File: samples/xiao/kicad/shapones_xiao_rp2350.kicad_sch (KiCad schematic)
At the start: 44 parts, among them Q1 PMOS, Q4 NMOS, SW1 POWER, SW10 MENU, SW2 A, SW3 B, SW4 SELECT, SW5 START, SW6 UP, SW7 DOWN, SW8 LEFT, SW9 RIGHT, U1 XIAO RP2350, U2 PCA9555D, U4 1.54''IPS-240x240, U5 TFCard, U6 74AHC1G04W5, U7 HT82V73A

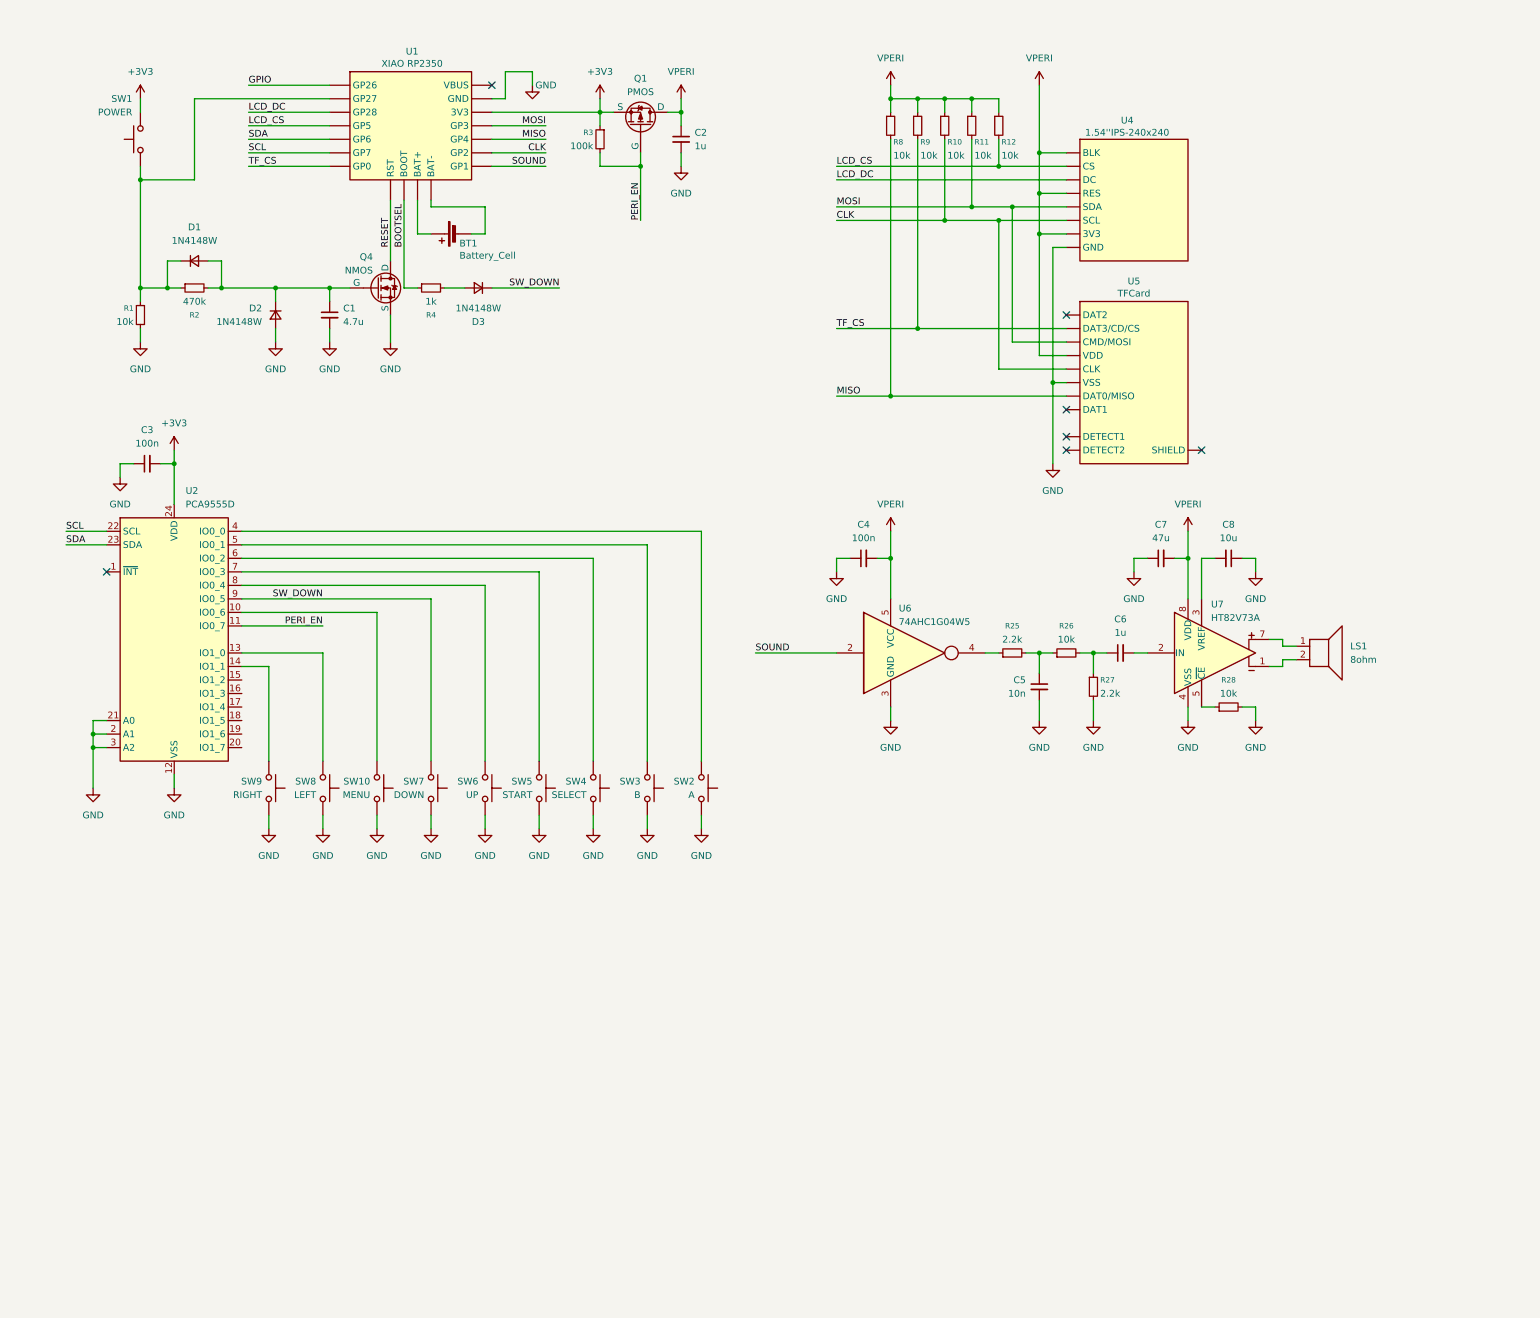
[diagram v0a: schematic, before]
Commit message: wip: PCB layout
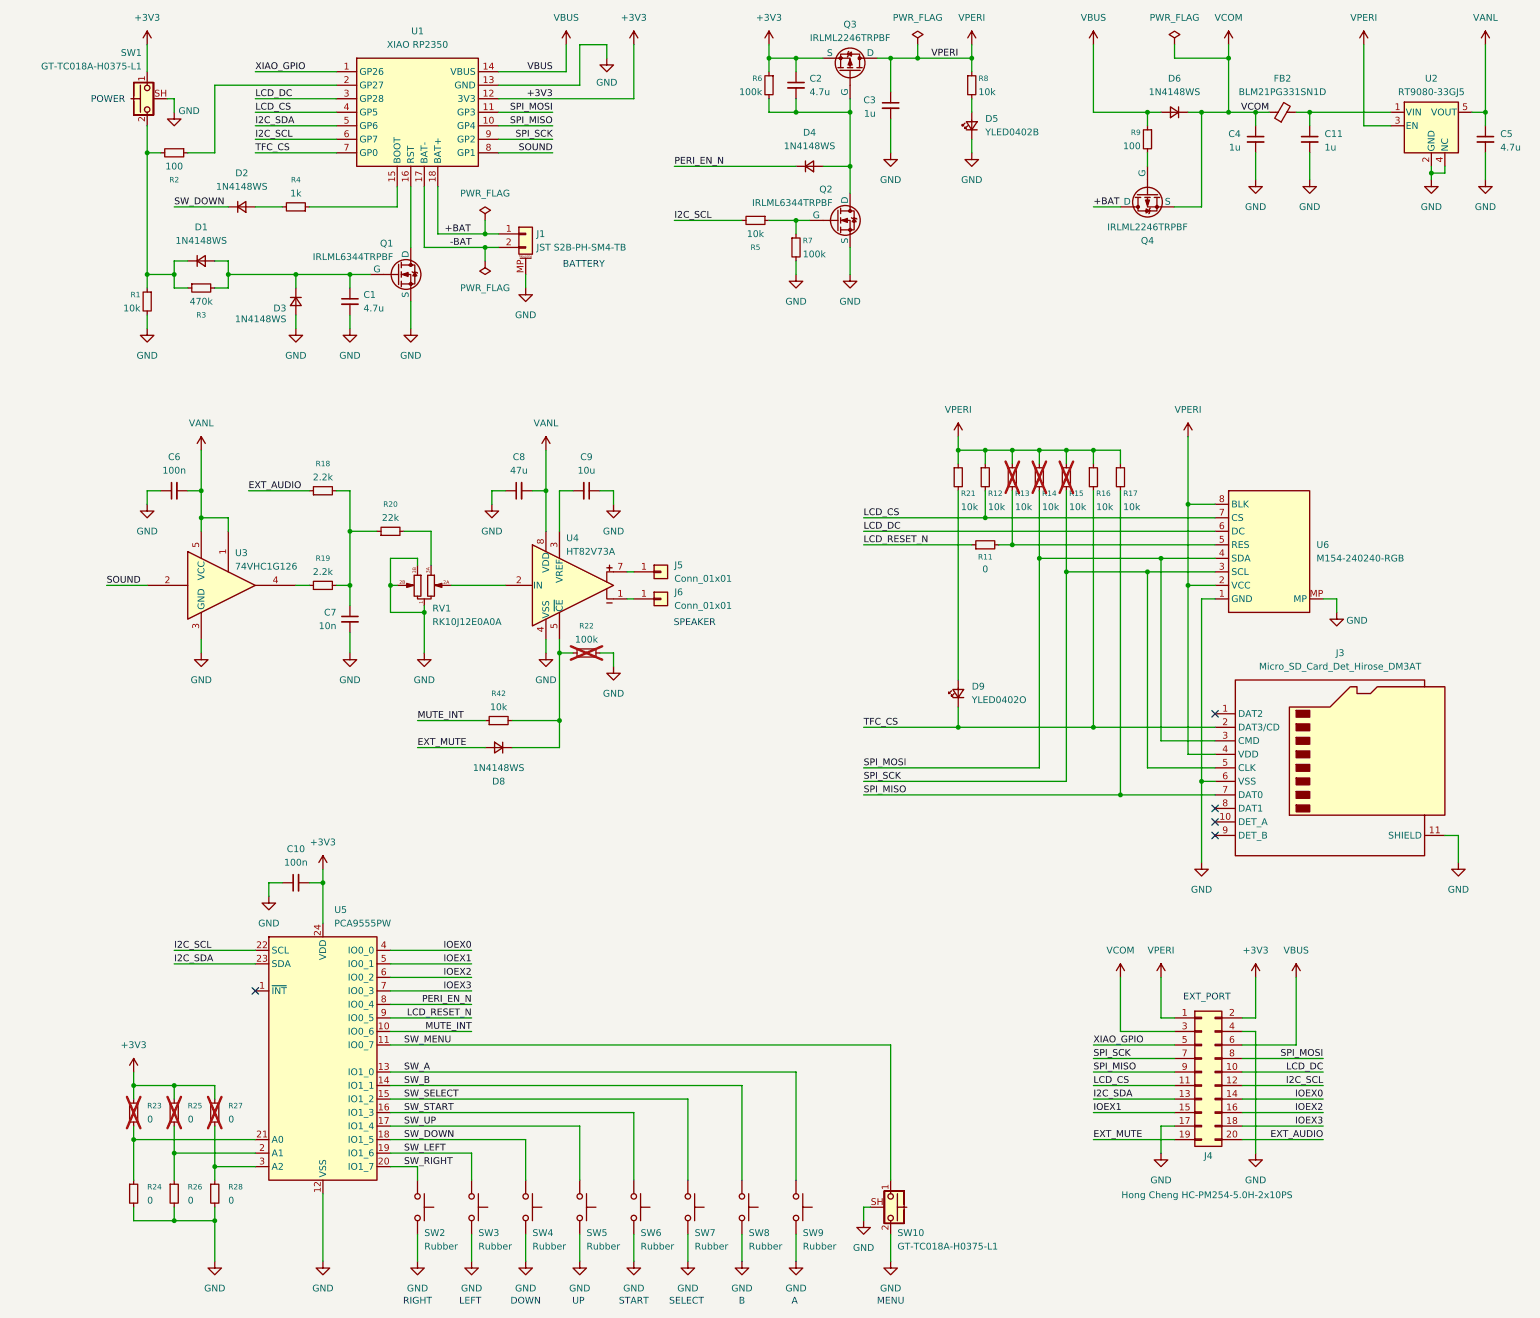
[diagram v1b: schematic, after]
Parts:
- removed BT1: Battery_Cell, symbol Device:Battery_Cell
- removed C6: 1u, symbol Device:C_Small
- removed LS1: 8ohm, symbol Device:Speaker
- removed SW1: POWER, symbol Switch:SW_Push
- removed SW10: MENU, symbol Switch:SW_Push
- removed SW2: A, symbol Switch:SW_Push
- removed SW3: B, symbol Switch:SW_Push
- removed SW4: SELECT, symbol Switch:SW_Push
- removed SW5: START, symbol Switch:SW_Push
- removed SW6: UP, symbol Switch:SW_Push
- removed SW7: DOWN, symbol Switch:SW_Push
- removed SW8: LEFT, symbol Switch:SW_Push
- removed SW9: RIGHT, symbol Switch:SW_Push
- removed U1: XIAO RP2350, symbol shpc_modules:RaspberryPiPico
- removed U2: PCA9555D, Package_SO:SOIC-24W_7.5x15.4mm_P1.27mm, symbol Interface_Expansion:PCA9555D
- removed U4: 1.54''IPS-240x240, symbol shpc_modules:RaspberryPiPico
- removed U5: TFCard, symbol shpc_modules:RaspberryPiPico
- removed U6: 74AHC1G04W5, Package_TO_SOT_SMD:SOT-553, symbol 74xGxx:74LVC1GU04DRL
- removed U7: HT82V73A, Package_SO:JEITA_SOIC-8_3.9x4.9mm_P1.27mm, symbol Amplifier_Audio:IS31AP4991-GRLS2
- added C11, C4: 1u, Capacitor_SMD:C_0402_1005Metric, symbol Device:C_Small
- added C2: 4.7u, Capacitor_SMD:C_0603_1608Metric, symbol Device:C_Small
- added C5: 4.7u, Capacitor_SMD:C_0402_1005Metric, symbol Device:C_Small
- added D4, D6, D8: 1N4148WS, Diode_SMD:D_SOD-323, symbol Device:D_Small
- added D5: YLED0402B, LED_SMD:LED_0402_1005Metric, symbol Device:LED_Small
- added D9: YLED0402O, LED_SMD:LED_0402_1005Metric, symbol Device:LED_Small
- added FB2: BLM21PG331SN1D, Inductor_SMD:L_Walsin_WLFM201209x, symbol Device:FerriteBead_Small
- added J1: JST S2B-PH-SM4-TB, Connector_JST:JST_PH_S2B-PH-SM4-TB_1x02-1MP_P2.00mm_Horizontal, symbol Connector_Generic_MountingPin:Conn_01x02_MountingPin
- added J3: Micro_SD_Card_Det_Hirose_DM3AT, Connector_Card:microSD_HC_Hirose_DM3AT-SF-PEJM5, symbol Connector:Micro_SD_Card_Det_Hirose_DM3AT
- added J4: Hong Cheng HC-PM254-5.0H-2x10PS, Connector_PinSocket_2.54mm:PinSocket_2x10_P2.54mm_Vertical_SMD, symbol Connector_Generic:Conn_02x10_Odd_Even
- added J5, J6: Conn_01x01, Connector_Wire:SolderWirePad_1x01_SMD_2x4mm, symbol Connector_Generic:Conn_01x01
- added Q2: IRLML6344TRPBF, Package_TO_SOT_SMD:SOT-23, symbol Simulation_SPICE:NMOS
- added Q4: IRLML2246TRPBF, Package_TO_SOT_SMD:SOT-23, symbol Simulation_SPICE:PMOS
- added R11, R23, R24, R25: 0, Resistor_SMD:R_0402_1005Metric, symbol Device:R_Small
- added R16, R21, R42, R5, R8: 10k, Resistor_SMD:R_0402_1005Metric, symbol Device:R_Small
- added R18: 2.2k, Resistor_SMD:R_0402_1005Metric, symbol Device:R_Small
- added R2, R9: 100, Resistor_SMD:R_0402_1005Metric, symbol Device:R_Small
- added R20: 22k, Resistor_SMD:R_0402_1005Metric, symbol Device:R_Small
- added R22, R7: 100k, Resistor_SMD:R_0402_1005Metric, symbol Device:R_Small
- added RV1: RK10J12E0A0A, shpc_mechanical:RK10J1xE, symbol shpc_mechanical:RK10J12E0A0A
- added SW1, SW10: GT-TC018A-H0375-L1, shpc_mechanical:GT-TC018A-H0375-L1, symbol Switch:SW_Push_Shielded
- added SW2, SW3, SW4, SW5, SW6, SW7, SW8, SW9: Rubber, shpc_mechanical:Rubber_Contact, symbol shpc_mechanical:Rubber_Contact
- added U1: XIAO RP2350, shpc_modules:XIAO RP2350, symbol shpc_modules:XIAO_RP2350
- added U2: RT9080-33GJ5, Package_TO_SOT_SMD:TSOT-23-5, symbol shpc_ic:RT9080-33GJ5
- added U3: 74VHC1G126, Package_TO_SOT_SMD:SOT-23-5, symbol shpc_ic:MC74VHC1G126DTT1G-TP
- added U4: HT82V73A, shpc_ic:SOIC-8_with_Thermal_Hole, symbol shpc_ic:HT82V73A
- added U5: PCA9555PW, Package_SO:TSSOP-24_4.4x7.8mm_P0.65mm, symbol Interface_Expansion:PCA9555PW
- added U6: M154-240240-RGB, shpc_modules:M154-240240-RGB, symbol shpc_modules:M154-240240-RGB
- C1: footprint (none) -> Capacitor_SMD:C_0603_1608Metric
- C10: renamed from C3; footprint (none) -> Capacitor_SMD:C_0402_1005Metric
- C3: renamed from C2; footprint (none) -> Capacitor_SMD:C_0402_1005Metric
- C6: renamed from C4; footprint (none) -> Capacitor_SMD:C_0402_1005Metric
- C7: renamed from C5; footprint (none) -> Capacitor_SMD:C_0402_1005Metric
- C8: renamed from C7; footprint (none) -> Capacitor_SMD:C_0603_1608Metric
- C9: renamed from C8; footprint (none) -> Capacitor_SMD:C_0603_1608Metric
- D1, D2, D3: value 1N4148W -> 1N4148WS; footprint (none) -> Diode_SMD:D_SOD-323; LCSC (none) -> C60580
- Q1: renamed from Q4; value NMOS -> IRLML6344TRPBF; footprint (none) -> Package_TO_SOT_SMD:SOT-23; LCSC (none) -> C53550
- Q3: renamed from Q1; value PMOS -> IRLML2246TRPBF; footprint (none) -> Package_TO_SOT_SMD:SOT-23; LCSC (none) -> C127272
- R1, R4: footprint (none) -> Resistor_SMD:R_0402_1005Metric
- R12: renamed from R8; footprint (none) -> Resistor_SMD:R_0402_1005Metric
- R13: renamed from R9; footprint (none) -> Resistor_SMD:R_0402_1005Metric; now not fitted
- R14: renamed from R10; footprint (none) -> Resistor_SMD:R_0402_1005Metric; now not fitted
- R15: renamed from R11; footprint (none) -> Resistor_SMD:R_0402_1005Metric; now not fitted
- R17: renamed from R12; footprint (none) -> Resistor_SMD:R_0402_1005Metric
- R19: renamed from R25; footprint (none) -> Resistor_SMD:R_0402_1005Metric
- R26, R28: value 10k -> 0; footprint (none) -> Resistor_SMD:R_0402_1005Metric
- R27: value 2.2k -> 0; footprint (none) -> Resistor_SMD:R_0402_1005Metric; now not fitted
- R3: renamed from R2; footprint (none) -> Resistor_SMD:R_0402_1005Metric
- R6: renamed from R3; footprint (none) -> Resistor_SMD:R_0402_1005Metric
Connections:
- net MISO is gone; now on net LCD_CS: R12.2
- net +3V3: now also R27.1, C2.1, J4.2 (Pin_2), R23.1, R25.1, SW1.1, U1.12 (3V3), U5.24 (VDD)
- net GND: now also D3.2 (A), R26.2, C11.2, C4.2, C5.2, D5.1 (K), J1.MP (MountPin), J3.11 (SHIELD), J3.6 (VSS), J4.17 (Pin_17), J4.4 (Pin_4), Q2.3 (S), R22.2, R24.2, R7.2, RV1.1, RV1.2B, RV1.3B, SW1.SH (B), SW10.2, SW10.SH (B), SW2.2, SW3.2, SW4.2, SW5.2, SW6.2, SW7.2, SW8.2, SW9.2, U1.13 (GND), U2.2 (GND), U2.4 (NC), U3.3 (GND), U4.4 (VSS), U5.12 (VSS), U6.1 (GND), U6.MP; no longer D2.2 (A), R27.2
- net LCD_CS: now also J4.11 (Pin_11), U1.4 (GP5), U6.7 (CS); no longer R17.2
- net LCD_DC: now also J4.10 (Pin_10), U1.3 (GP28), U6.6 (DC)
- net SOUND: now also U1.8 (GP1), U3.2
- net SW_DOWN: now also D2.1 (K), SW4.1, U5.18 (IO1_5); no longer D3.1 (K)
- net VPERI: now also J3.4 (VDD), J4.1 (Pin_1), R16.1, R21.1, R8.1, U2.3 (EN), U6.2 (VCC), U6.8 (BLK); no longer C6.2, C8.2
- net at D1.1 (K), R1.1, R3.1: now also R2.2, SW1.2
- net at R4.2: now also D2.2 (A); no longer D3.2 (A)
- net at R28.1: now also R27.2, U5.3 (A2)
- net at C9.2: now also U4.3 (VREF)
- net at C1.1, D1.2 (A), Q1.2 (G)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: now also D3.1 (K); no longer D2.1 (K)
- net at C7.1, R19.2: now also R18.2, R20.1; no longer R26.1
- net at R19.1: now also U3.4
- net BOOTSEL: no longer names the net of R4.1
- net BOOTSEL: now also U1.15 (BOOT)
- net CLK renamed SPI_MOSI
- net SPI_MOSI: now also J3.3 (CMD), J4.8 (Pin_8), U1.11 (GP3), U6.4 (SDA)
- net MOSI renamed SPI_SCK
- net SPI_SCK: now also J3.5 (CLK), J4.7 (Pin_7), U1.9 (GP2), U6.3 (SCL)
- net PERI_EN: no longer names the net of Q3.2 (G), R6.2
- net PERI_EN: now also C2.2, D4.2 (A), Q2.1 (D)
- net RESET: no longer names the net of Q1.1 (D)
- net RESET: now also U1.16 (RST)
- net TF_CS: no longer names the net of R13.2
- net TF_CS: now also R11.2, U6.5 (RES)
- new net: J6.1 (Pin_1), U4.1
- new net: RV1.2A, U4.2 (IN)
- new net: D8.1 (K), R22.1, R42.2, U4.5 (~{CE})
- new net: J5.1 (Pin_1), U4.7
- new net: Q2.2 (G), R5.1, R7.1
- new net: R20.2, RV1.3A
- new net: C11.1, FB2.2, U2.1 (VIN)
- new net: D9.2 (A), R21.2
- new net: R23.2, R24.1, U5.21 (A0)
- new net: Q4.2 (G), R9.2
- new net: R25.2, R26.1, U5.2 (A1)
- new net: D5.2 (A), R8.2
- new net: R2.1, U1.2 (GP27)
- new net +BAT: J1.1 (Pin_1), Q4.1 (D), U1.18 (BAT+)
- new net -BAT: J1.2 (Pin_2), U1.17 (BAT-)
- new net EXT_AUDIO: J4.20 (Pin_20), R18.1
- new net EXT_MUTE: D8.2 (A), J4.19 (Pin_19)
- new net I2C_SCL: J4.12 (Pin_12), R5.2, U1.6 (GP7), U5.22 (SCL)
- new net I2C_SDA: J4.13 (Pin_13), U1.5 (GP6), U5.23 (SDA)
- new net IOEX0: J4.14 (Pin_14), U5.4 (IO0_0)
- new net IOEX1: J4.15 (Pin_15), U5.5 (IO0_1)
- new net IOEX2: J4.16 (Pin_16), U5.6 (IO0_2)
- new net IOEX3: J4.18 (Pin_18), U5.7 (IO0_3)
- new net LCD_RESET_N: R11.1, U5.9 (IO0_5)
- new net MUTE_INT: R42.1, U5.10 (IO0_6)
- new net PERI_EN_N: D4.1 (K), U5.8 (IO0_4)
- new net SPI_MISO: J3.7 (DAT0), J4.9 (Pin_9), R17.2, U1.10 (GP4)
- new net SW_A: SW9.1, U5.13 (IO1_0)
- new net SW_B: SW8.1, U5.14 (IO1_1)
- new net SW_LEFT: SW3.1, U5.19 (IO1_6)
- new net SW_MENU: SW10.1, U5.11 (IO0_7)
- new net SW_RIGHT: SW2.1, U5.20 (IO1_7)
- new net SW_SELECT: SW7.1, U5.15 (IO1_2)
- new net SW_START: SW6.1, U5.16 (IO1_3)
- new net SW_UP: SW5.1, U5.17 (IO1_4)
- new net TFC_CS: D9.1 (K), J3.2 (DAT3/CD), R16.2, U1.7 (GP0)
- new net VANL: C5.1, C6.2, C8.2, U2.5 (VOUT), U3.1, U3.5 (VCC), U4.8 (VDD)
- new net VBUS: D6.2 (A), J4.6 (Pin_6), R9.1, U1.14 (VBUS)
- new net VCOM: C4.1, D6.1 (K), FB2.1, J4.3 (Pin_3), Q4.3 (S)
- new net XIAO_GPIO: J4.5 (Pin_5), U1.1 (GP26)
- no-connect marks 7 -> 5
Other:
- note added: "A"
- note added: "B"
- note added: "BATTERY"
- note added: "DOWN"
- note added: "EXT_PORT"
- note added: "LEFT"
- note added: "MENU"
- note added: "POWER"
- note added: "RIGHT"
- note added: "SELECT"
- note added: "SPEAKER"
- note added: "START"
- note added: "UP"
- moved on the sheet: C1, C10, C3, C6, C7, C8, C9, D1, Q1, Q3, R1, R12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
